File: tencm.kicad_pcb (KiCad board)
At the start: 2 copper layers, 27.9 x 63.5 mm, 4 parts

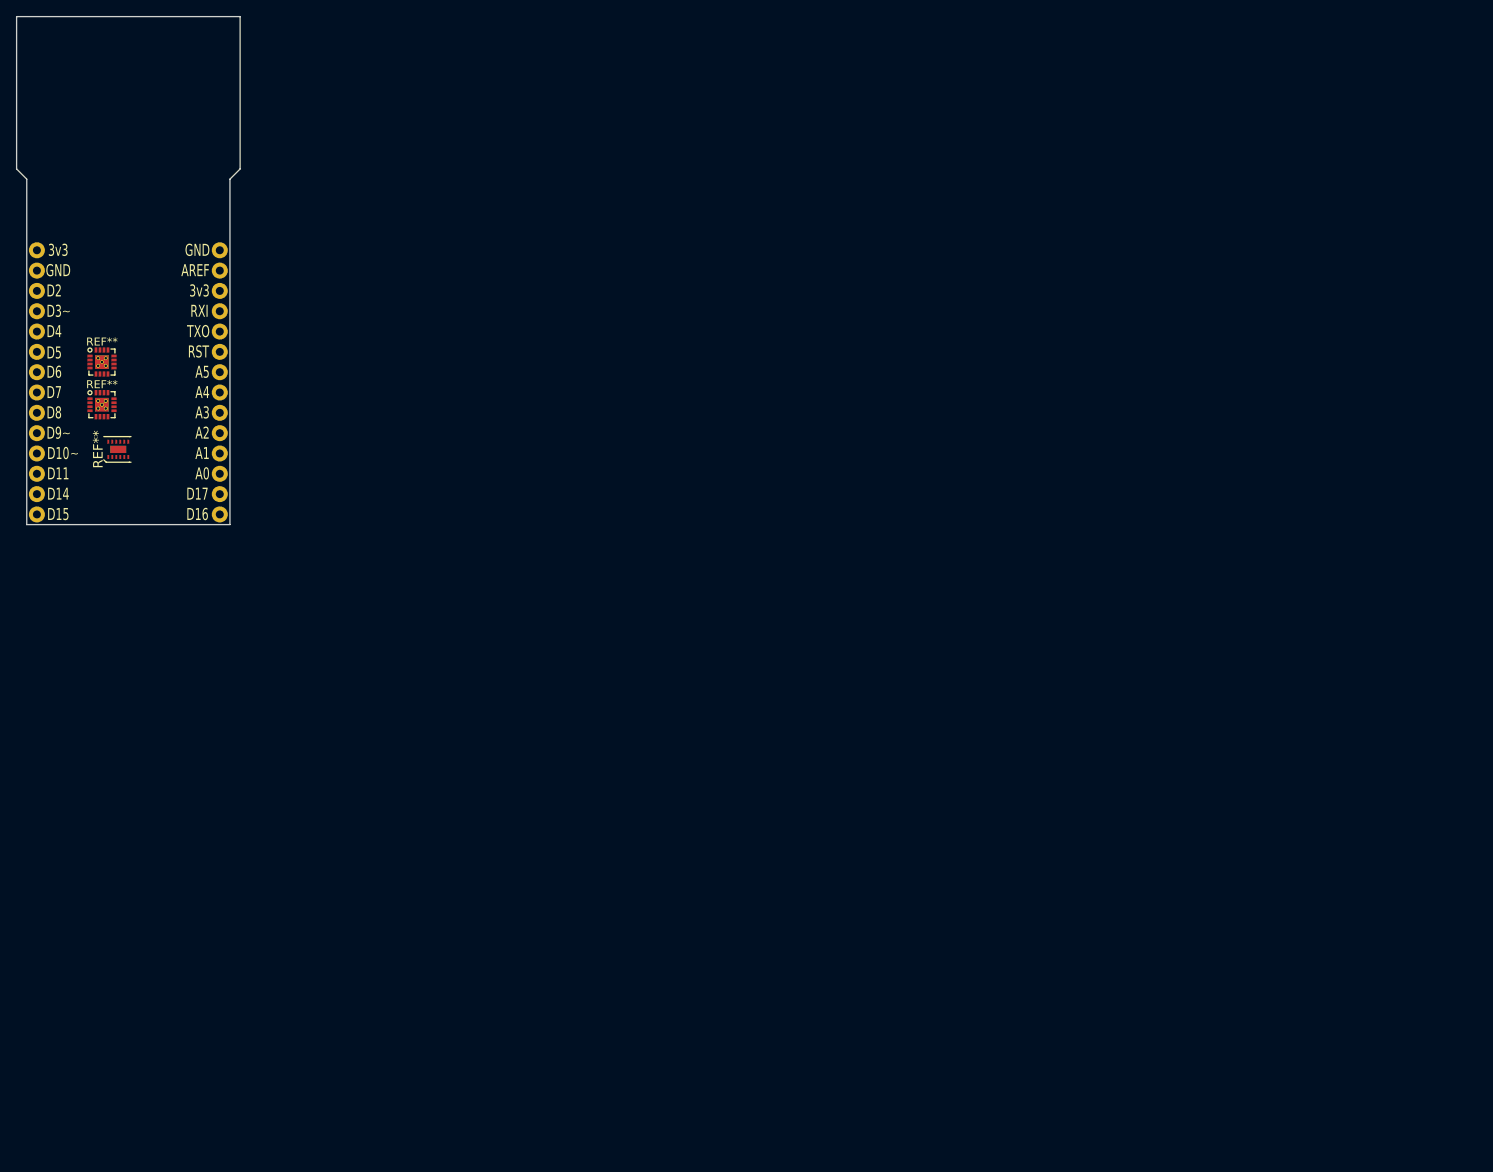
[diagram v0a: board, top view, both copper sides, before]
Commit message: initiial layout
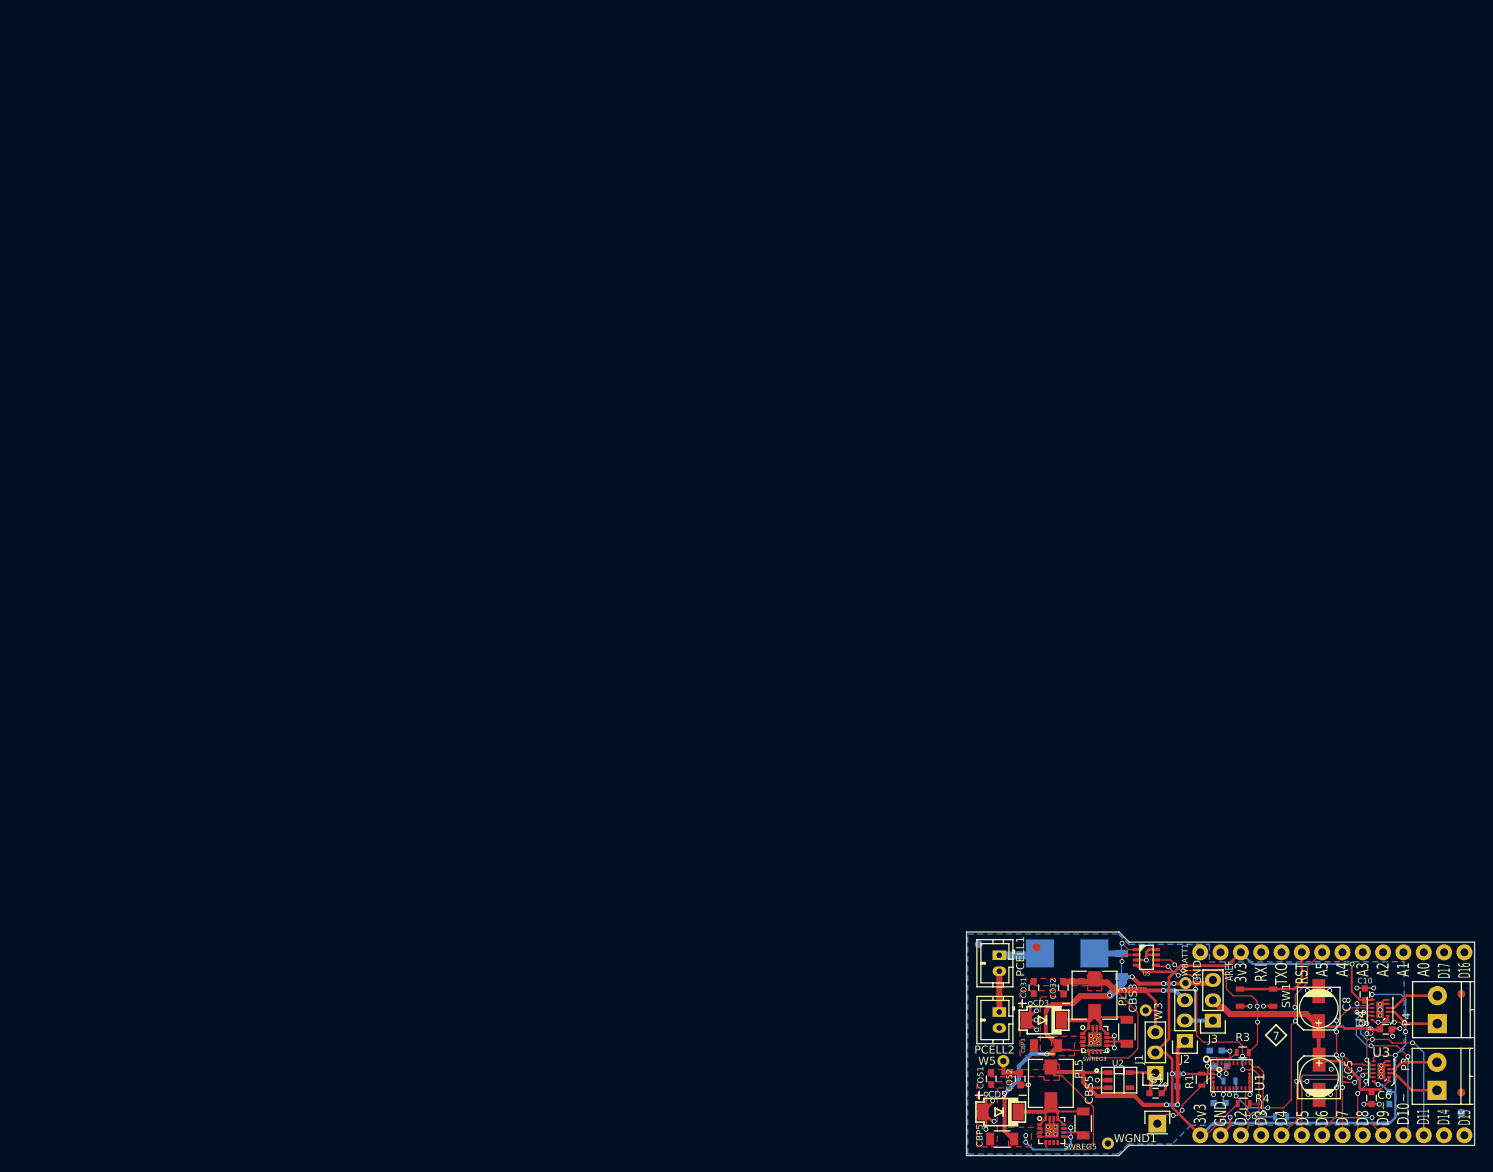
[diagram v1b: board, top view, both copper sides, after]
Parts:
- removed REF** (x2): QFN16, customFootprints:QFN16_TS30013
- removed REF**: DIP-30_1, customFootprints:FIO_DIP
- removed REF**: SOIC-12, customFootprints:SOIC-12
- added C1: 100nF, Capacitors_SMD:C_0603, B.Cu at (142.6, 70.7)
- added C10: 0.1uF, Capacitors_SMD:C_0603, F.Cu at (166.0, 60.0)
- added C11: 100n, Capacitors_SMD:C_0603, B.Cu at (147.8, 73.5)
- added C2: 4.7nF, Capacitors_SMD:C_0603, B.Cu at (147.3, 67.0)
- added C3: 100nF, Capacitors_SMD:C_0603, B.Cu at (148.0, 69.0)
- added C4: 1u, Capacitors_SMD:C_0603, F.Cu at (139.8, 72.3)
- added C5: 100uF, Capacitors_SMD:c_elec_5x5.3, F.Cu at (160.3, 70.4)
- added C6: 0.1uF, Capacitors_SMD:C_0603, F.Cu at (166.8, 72.9)
- added C7: 0.1uF, Capacitors_SMD:C_0603, B.Cu at (169.1, 73.0)
- added C8: 100uF, Capacitors_SMD:c_elec_5x5.3, F.Cu at (160.2, 61.8)
- added C9: 0.1uF, Capacitors_SMD:C_0603, F.Cu at (168.6, 64.4)
- added CBP3: GMK316F106ZL-T, Capacitors_SMD:C_1206, F.Cu at (126.1, 66.4)
- added CBP5: GMK316F106ZL-T, Capacitors_SMD:C_1206, F.Cu at (120.7, 78.1)
- added CBS3: GMK316F106ZL-T, Capacitors_SMD:C_1206, F.Cu at (136.2, 64.7)
- added CBS5: GMK316F106ZL-T, Capacitors_SMD:C_1206, F.Cu at (130.8, 76.1)
- added CD3: PMEG4050EP, gsg-modules:SOD128, F.Cu at (125.9, 63.2)
- added CD5: PMEG4050EP, gsg-modules:SOD128, F.Cu at (120.5, 74.7)
- added CO31: CC0603MRX5R5BB226, Capacitors_SMD:C_0603, F.Cu at (124.6, 59.2)
- added CO32: CC0603MRX5R5BB226, Capacitors_SMD:C_0603, F.Cu at (128.3, 59.2)
- added CO51: CC0603MRX5R5BB226, Capacitors_SMD:C_0603, F.Cu at (119.3, 70.5)
- added CO52: CC0603MRX5R5BB226, Capacitors_SMD:C_0603, F.Cu at (122.9, 70.5)
- added F1: MINISMDC200F-2, Resistors_SMD:R_1812_HandSoldering, B.Cu at (128.8, 54.9)
- added FID1: Fiducial_1mm_Dia_2.54mm_Outer_CopperTop, Fiducials:Fiducial_1mm_Dia_2.54mm_Outer_CopperTop, F.Cu at (125.0, 54.1)
- added FID2: Fiducial_1mm_Dia_2.54mm_Outer_CopperTop, Fiducials:Fiducial_1mm_Dia_2.54mm_Outer_CopperTop, F.Cu at (178.1, 59.9)
- added FID3: Fiducial_1mm_Dia_2.54mm_Outer_CopperTop, Fiducials:Fiducial_1mm_Dia_2.54mm_Outer_CopperTop, F.Cu at (178.1, 72.3)
- added FID4: Fiducial_1mm_Dia_2.54mm_Outer_CopperTop, Fiducials:Fiducial_1mm_Dia_2.54mm_Outer_CopperTop, B.Cu at (117.7, 53.7)
- added FID5: Fiducial_1mm_Dia_2.54mm_Outer_CopperTop, Fiducials:Fiducial_1mm_Dia_2.54mm_Outer_CopperTop, B.Cu at (178.1, 74.8)
- added FID6: Fiducial_1mm_Dia_2.54mm_Outer_CopperTop, Fiducials:Fiducial_1mm_Dia_2.54mm_Outer_CopperTop, B.Cu at (117.9, 74.8)
- added J1: CONN_01X03, Pin_Headers:Pin_Header_Straight_1x03, F.Cu at (139.8, 69.8)
- added J2: CONN_01X03, Pin_Headers:Pin_Header_Straight_1x03, F.Cu at (143.5, 65.8)
- added J3: CONN_01X03, Pin_Headers:Pin_Header_Straight_1x03, F.Cu at (147.0, 63.3)
- added P1: FIO_HEADER, customFootprints:FIO_DIP, F.Cu at (178.4, 77.6)
- added P2: CONN_01X01, Pin_Headers:Pin_Header_Straight_1x01, F.Cu at (140.1, 76.2)
- added P3: 1984617, Terminal_Blocks:TerminalBlock_Pheonix_PT-3.5mm_2pol, F.Cu at (175.0, 72.0)
- added P4: 1984617, Terminal_Blocks:TerminalBlock_Pheonix_PT-3.5mm_2pol, F.Cu at (175.1, 63.7)
- added PCELL1: S2B-PH-K-S(LF)(SN), Connectors_JST_PH:Connectors_JST_B2B-PH-K, F.Cu at (120.3, 55.1)
- added PCELL2: S2B-PH-K-S(LF)(SN), Connectors_JST_PH:Connectors_JST_B2B-PH-K, F.Cu at (120.3, 62.2)
- added PL3: 4.7uH, customFootprints:L_5040, F.Cu at (132.2, 60.1)
- added PL5: 4.7uH, customFootprints:L_5040, F.Cu at (126.7, 71.1)
- added R1: 10k, Resistors_SMD:R_0603, F.Cu at (145.6, 70.7)
- added R2: 10k, Resistors_SMD:R_0603, B.Cu at (149.1, 70.8)
- added R3: 4.7k, Resistors_SMD:R_0603, F.Cu at (150.7, 67.2)
- added R4: 4.7k, Resistors_SMD:R_0603, F.Cu at (150.8, 73.7)
- added R5: 100, Resistors_SMD:R_0603, B.Cu at (155.5, 75.3)
- added RS1: 0.1, MF_Passives:MF_Passives-R1206, B.Cu at (135.6, 56.3)
- added SW1: PTS810, customFootprints:BTN_PTS_810, F.Cu at (152.5, 60.4)
- added SWREG3: TS30013, customFootprints:QFN16_TS30013, F.Cu at (132.2, 65.6)
- added SWREG5: TS30013-M050QFNR, customFootprints:QFN16_TS30013, F.Cu at (126.8, 77.0)
- added U1: BNO055, customFootprints:BNO055-SOIC, F.Cu at (149.3, 70.2)
- added U2: TLV70212DBV, MF_IC_Power:MF_IC_Power-SOT-23-5, F.Cu at (135.3, 70.7)
- added U3: DRV8839, customFootprints:SOIC-12-DRV8839, F.Cu at (168.0, 69.6)
- added U4: DRV8839, customFootprints:SOIC-12-DRV8839, F.Cu at (167.9, 61.9)
- added U5: INA219BIDCNT, w_smd_trans:sot23-8, F.Cu at (138.7, 55.4)
- added W3: TEST_1P, Measurement_Points:Measurement_Point_Round-TH_Small, F.Cu at (138.6, 62.0)
- added W5: TEST_1P, Measurement_Points:Measurement_Point_Round-TH_Small, F.Cu at (120.8, 68.3)
- added WBATT1: TEST_1P, Measurement_Points:Measurement_Point_Round-TH_Small, F.Cu at (143.6, 58.6)
- added WGND1: TEST_1P, Measurement_Points:Measurement_Point_Round-TH_Small, F.Cu at (133.9, 78.6)
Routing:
- net 3v3_SEL: track 0.00 -> 173.9 mm, vias 0 -> 12
- net VBATT: track 0.00 -> 79.2 mm, vias 0 -> 15
- net GGND: track 0.00 -> 66.2 mm, vias 0 -> 30
- net 5v0: track 0.00 -> 58.3 mm, vias 0 -> 2
- net 3v3_SW: track 0.00 -> 47.7 mm, vias 0 -> 1
- net VMOT: track 0.00 -> 43.5 mm
- net SDA: track 0.00 -> 36.1 mm, vias 0 -> 6
- net SCL: track 0.00 -> 33.4 mm, vias 0 -> 6
- net GRST: track 0.00 -> 31.0 mm, vias 0 -> 4
- net M2I2: track 0.00 -> 25.4 mm, vias 0 -> 5
- net M2I1: track 0.00 -> 22.1 mm, vias 0 -> 3
- net M2E: track 0.00 -> 20.6 mm, vias 0 -> 4
- net Net-(CBS3-Pad1): track 0.00 -> 18.7 mm
- net M1I1: track 0.00 -> 18.6 mm, vias 0 -> 4
- net Net-(CBS5-Pad1): track 0.00 -> 18.0 mm
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- added copper zone on F.Cu, net 3v3_SW
- added copper zone on F.Cu, net 5v0
- added copper zone on B.Cu, net GGND
- added copper zone on F.Cu, net GGND
- added copper zone on F.Cu, net VBATT
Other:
- board size 27.9 x 63.5 mm -> 63.5 x 27.9 mm
- net class Default: clearance 0.2 -> 0.14
- net class pwr added: clearance 0.14, trace_width 1, via_dia 0.6, via_drill 0.4
- rule trace_clearance: 0.2 -> 0.14
- rule trace_min: 0.2 -> 0.14
- board text added: "7"
